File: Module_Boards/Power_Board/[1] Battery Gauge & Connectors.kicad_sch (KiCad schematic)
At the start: 6 parts, among them U1 MAX17262REWL+T

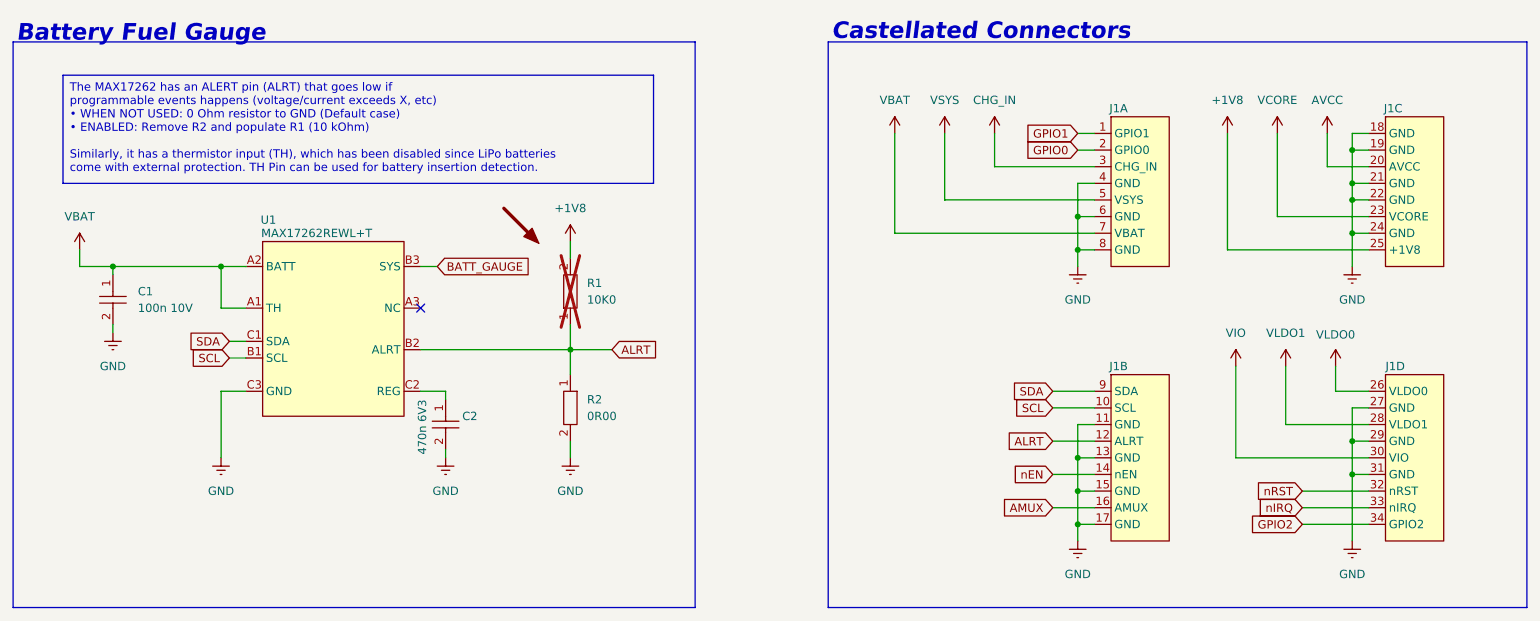
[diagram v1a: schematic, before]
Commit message: Push with updated readme
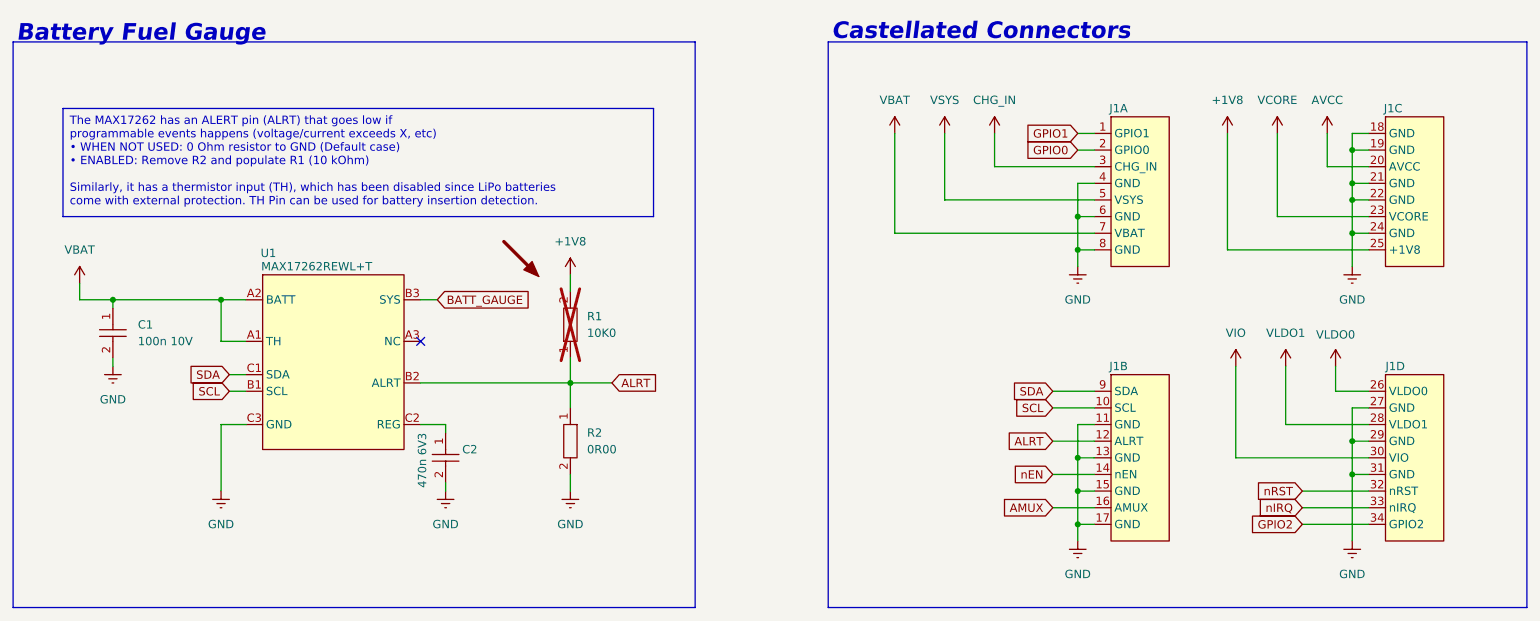
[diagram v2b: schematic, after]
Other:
- moved on the sheet: C1, C2, R1, R2, U1
